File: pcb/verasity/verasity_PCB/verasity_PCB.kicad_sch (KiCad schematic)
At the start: 98 parts, among them U10 F7, U11 F8, U12 F9, U13 F10, U14 F11, U15 F12, U16 PR_SC, U17 SCRLC, U18 PoBr, U19 `, U2 ESC, U20 1, U21 2, U22 3, U23 4, U24 5, U25 6, U26 7, U27 8, U28 9, U29 0, U3 custom1, U30 -, U31 =, U32 BackSp, U33 Ins, U34 Home, U35 PaUp, U36 Tab, U37 Q, U38 W, U39 E, U4 F1, U40 R, U41 T, U42 Y, U43 U, U44 I, U45 O, U46 P, U47 [, U48 ], U49 \, U5 F2, U50 Del, U51 End, U52 PaDo, U53 Caps, U54 A, U55 S, U56 D, U57 F, U58 G, U59 H, U6 F3, U60 J, U61 K, U62 L, U63 ;, U64 ", U65 Ent, U66 LShif, U67 Z, U68 X, U69 C, U7 F4, U70 V, U71 B, U72 N, U73 M, U74 <, U75 >, U76 ?, U77 Custom, U78 RShif, U79 ArUp, U8 F5, U80 LCrtl, U81 LSuper, U82 LAlt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

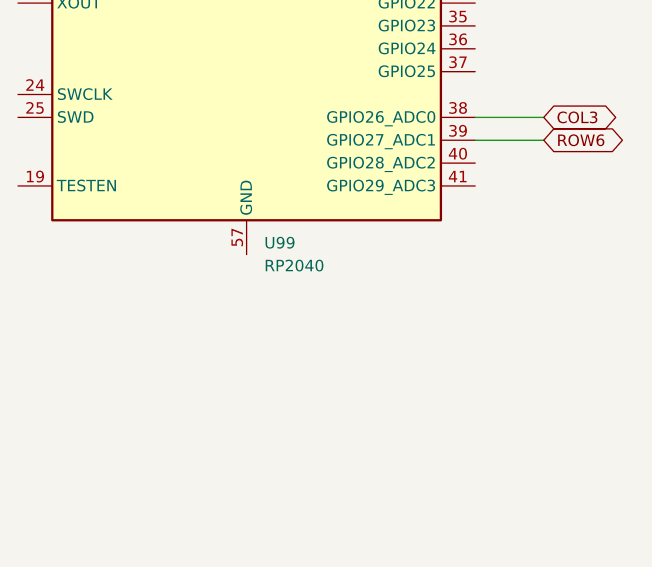
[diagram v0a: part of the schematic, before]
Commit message: cc
Signed-off-by: bornav <borna.vincek1@gmail.com>
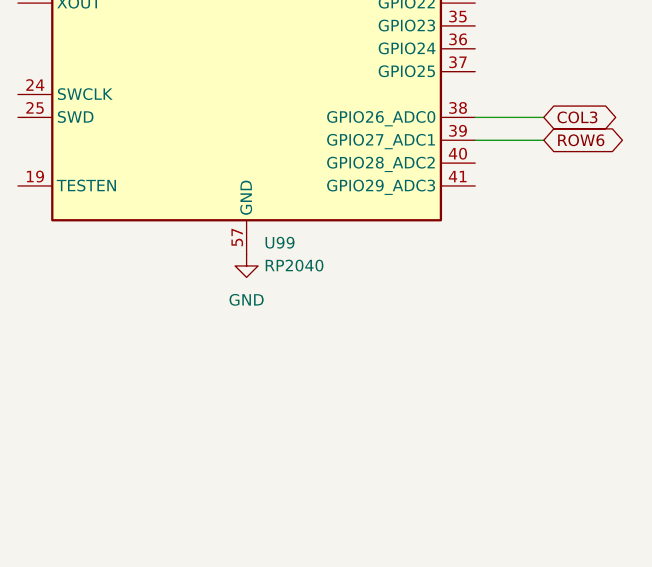
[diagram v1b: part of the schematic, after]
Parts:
- U99: footprint waveshare:waveshare-rp2040-zero -> waveshare:waveshare-rp2040-zero_no_inner
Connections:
- net GND: now reaches U99.57 (GND)
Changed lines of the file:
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@@
+    )
+  )
+  (symbol (lib_id "power:GND") (at -144.78 246.38 0) (unit 1)
+    (in_bom yes) (on_board yes) (dnp no) (fields_autoplaced)
+    (property "Reference" "#PWR01" (at -144.78 252.73 0)
+      (effects (font (size 1.27 1.27)) hide)
+    )
+    (property "Value" "GND" (at -144.78 251.46 0)
+      (effects (font (size 1.27 1.27)))
+    )
+    (property "Footprint" "" (at -144.78 246.38 0)
+      (effects (font (size 1.27 1.27)) hide)
+    )
+    (property "Datasheet" "" (at -144.78 246.38 0)
+      (effects (font (size 1.27 1.27)) hide)
+    )
+    (pin "1")
+    (instances
+      (project "verasity_PCB"
+        (path "/eb9e929c-804a-48fb-9333-213839b64271"
+          (reference "#PWR01") (unit 1)
+        )
+      )
     )
   )
@@
       (effects (font (size 1.27 1.27)) (justify left))
     )
-    (property "Footprint" "waveshare:waveshare-rp2040-zero" (at -144.78 200.66 0)
-      (effects (font (size 1.27 1.27)) hide)
-    )
+    (property "Footprint" "waveshare:waveshare-rp2040-zero_no_inner" (at -144.78 200.66 0)
+      (effects (font (size 1.27 1.27)) hide)
+    )

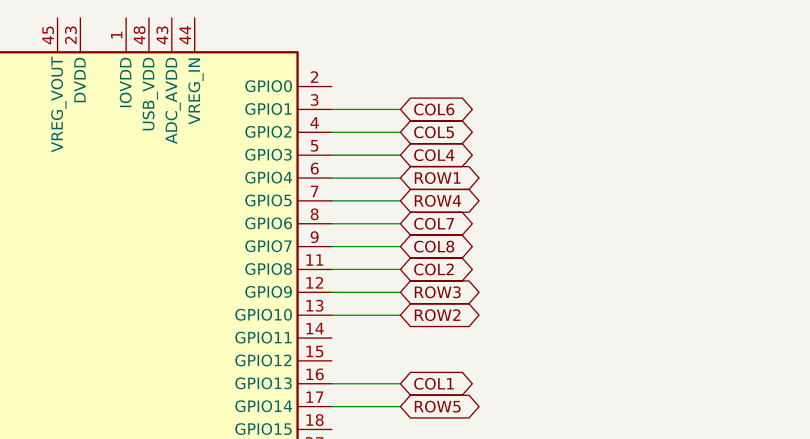
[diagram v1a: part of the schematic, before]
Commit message: prerelease
Signed-off-by: bornav <borna.vincek1@gmail.com>
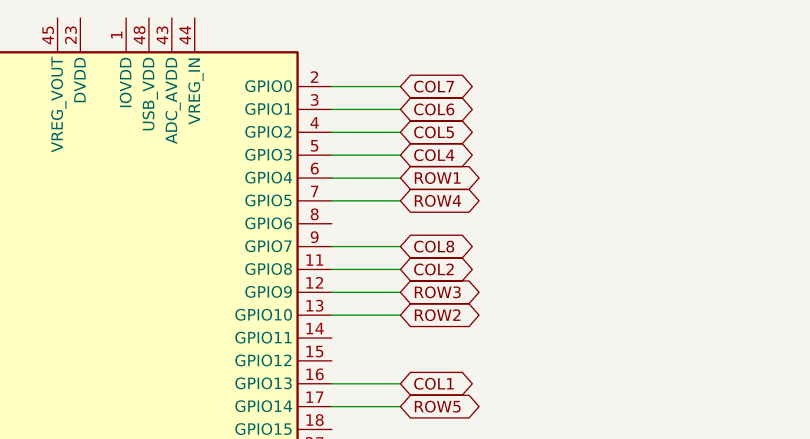
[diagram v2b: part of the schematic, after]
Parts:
- U99: footprint waveshare:waveshare-rp2040-zero_no_inner -> waveshare:waveshare-rp2040-pad_solder_with_cutout
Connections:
- net COL7: now also U99.2 (GPIO0); no longer U99.8 (GPIO6)
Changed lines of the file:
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@@
     (stroke (width 0) (type default))
   )
-  (wire (pts (xy -119.38 177.8) (xy -111.76 177.8))
-    (stroke (width 0) (type default))
-  )
   (wire (pts (xy -111.76 187.96) (xy -119.38 187.96))
     (stroke (width 0) (type default))
@@
     (stroke (width 0) (type default))
   )
+  (wire (pts (xy -119.38 162.56) (xy -111.76 162.56))
+    (stroke (width 0) (type default))
+  )
   (wire (pts (xy 135.89 254) (xy 135.89 262.89))
     (stroke (width 0) (type default))
@@
     )
   )
-  (global_label "COL7" (shape bidirectional) (at -111.76 177.8 0)
+  (global_label "COL7" (shape bidirectional) (at -111.76 162.56 0)
     (effects (font (size 1.27 1.27)) (justify left))
-    (property "Intersheetrefs" "${INTERSHEET_REFS}" (at -111.76 177.8 0)
+    (property "Intersheetrefs" "${INTERSHEET_REFS}" (at -111.76 162.56 0)
       (effects (font (size 1.27 1.27)) hide)
     )
@@
       (effects (font (size 1.27 1.27)) (justify left))
     )
-    (property "Footprint" "waveshare:waveshare-rp2040-zero_no_inner" (at -144.78 200.66 0)
+    (property "Footprint" "waveshare:waveshare-rp2040-pad_solder_with_cutout" (at -144.78 200.66 0)
       (effects (font (size 1.27 1.27)) hide)
     )
